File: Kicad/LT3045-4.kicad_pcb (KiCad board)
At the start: 4 copper layers, 100 x 50 mm, 26 parts, among them J1 Conn_Coaxial_Power, J2 Conn_Coaxial_Power, U1 LT3042, U2 LT3042, U3 LT3042, U4 LT3042

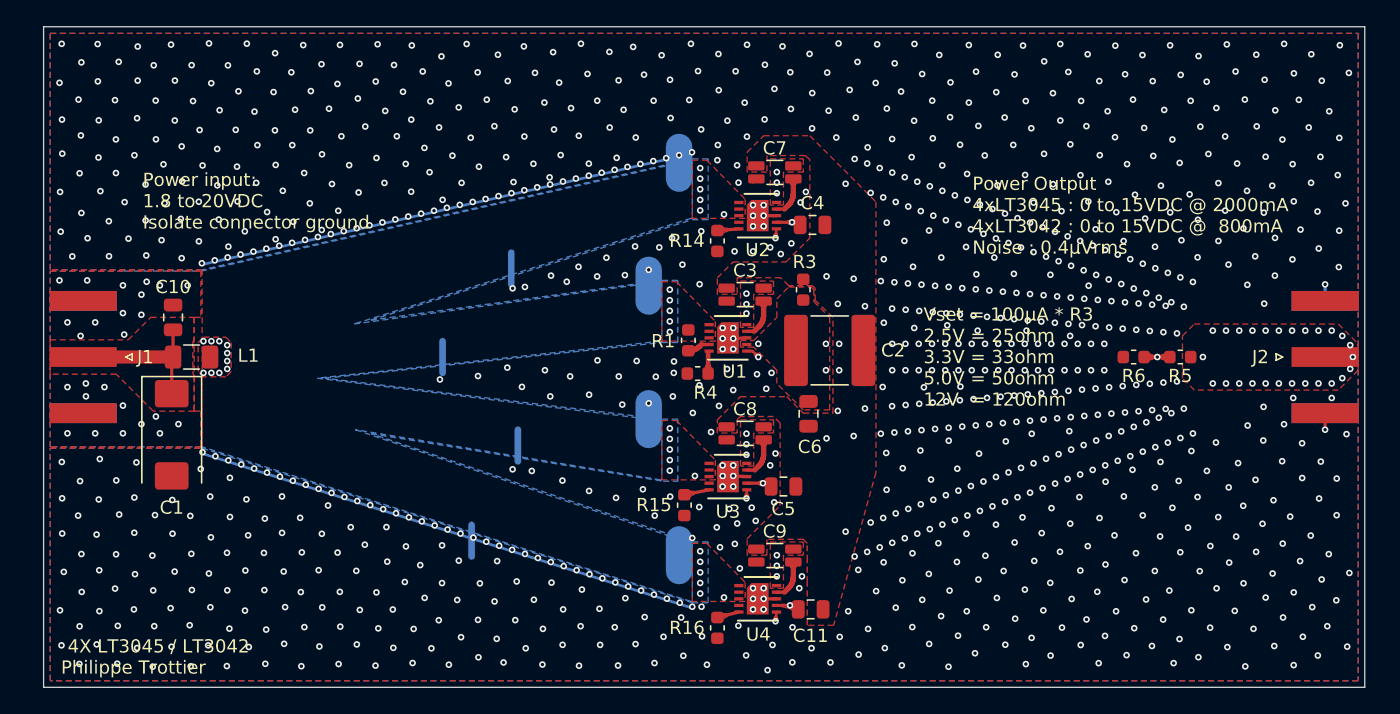
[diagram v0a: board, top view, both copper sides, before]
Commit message: Lost revision :(
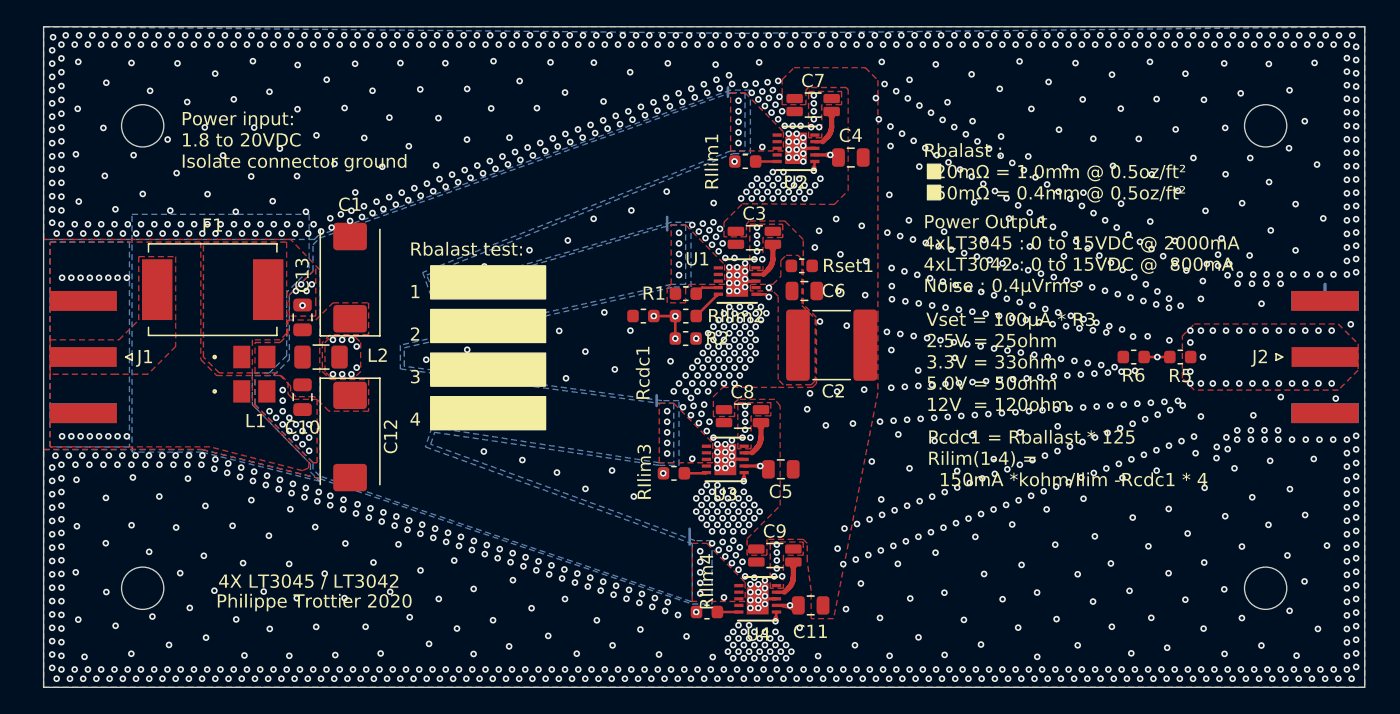
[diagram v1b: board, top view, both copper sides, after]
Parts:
- added C12: 22µF 35V, Capacitor_Tantalum_SMD:CP_EIA-7343-30_AVX-N, F.Cu at (23.2, 31.0)
- added C13: 4.7µF 35V, Capacitor_SMD:C_0805_2012Metric, F.Cu at (19.6, 22.0)
- added F1: 4A, Fuse:Fuse_Bourns_MF-SM_9.5x6.71mm, F.Cu at (12.8, 19.9)
- added L1: DLW5BTH101TQ2L, Transformer_SMD:CMC_DLW5BTH, F.Cu at (15.9, 26.3)
- added MH1: MountingHole_Pad, MountingHole:MountingHole_3.2mm_M3, F.Cu at (92.5, 7.50)
- added MH2: MountingHole_Pad, MountingHole:MountingHole_3.2mm_M3, F.Cu at (92.5, 42.5)
- added MH3: MountingHole_Pad, MountingHole:MountingHole_3.2mm_M3, F.Cu at (7.50, 7.50)
- added MH4: MountingHole_Pad, MountingHole:MountingHole_3.2mm_M3, F.Cu at (7.50, 42.5)
- added R2: 16.5k, Resistor_SMD:R_0603_1608Metric, F.Cu at (48.6, 23.6)
- added Rcdc1: Rcdc, Resistor_SMD:R_0603_1608Metric, F.Cu at (45.4, 21.9)
- RIlim1: renamed from R14; value 0 -> 287
- RIlim2: renamed from R4; value 0 -> 287
- RIlim3: renamed from R15; value 0 -> 287
- RIlim4: renamed from R16; value 0 -> 287
- moved C1 18.0 mm to (23.2, 19.0), turned to 90 degrees
- moved C10 11.5 mm to (19.6, 28.0), turned to 270 degrees
- moved L2 9.80 mm to (21.0, 25.0)
- moved C6 9.31 mm to (57.6, 20.0), turned to 0 degrees
- moved RIlim1 6.37 mm to (53.1, 10.2), turned to 180 degrees
- moved U2 5.87 mm to (57.0, 9.20)
- moved C7 5.87 mm to (58.2, 5.92)
- moved C4 5.87 mm to (61.1, 9.90)
- moved RIlim2 4.44 mm to (48.6, 21.9)
- moved U1 4.36 mm to (52.5, 19.2)
- moved C3 4.36 mm to (53.8, 16.0)
- moved R1 3.54 mm to (48.6, 20.2), turned to 180 degrees
- moved RIlim3 2.54 mm to (47.7, 33.8), turned to 180 degrees
- moved Rset1 1.80 mm to (57.4, 18.1), turned to 0 degrees
- moved RIlim4 1.44 mm to (50.2, 44.3), turned to 180 degrees
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- renumbered L1 to L2, R3 to Rset1
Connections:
- J1 pad 1: Net-(C1-Pad1) -> Net-(F1-Pad2)
- J1 pad 2: GND -> Net-(J1-Pad2)
- RIlim1 pad 2: GND -> /ILim
- RIlim2 pad 2: GND -> /ILim
- RIlim3 pad 2: GND -> /ILim
- RIlim4 pad 2: GND -> /ILim
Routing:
- net GND: track 105.6 -> 9.51 mm, vias 1093 -> 1604
- net /ILim: track 0.00 -> 41.6 mm, vias 0 -> 6
- net Net-(C1-Pad1): track 11.7 -> 0.00 mm
- net /VOUT: track 141.8 -> 131.5 mm, vias 38 -> 57
- net Net-(C11-Pad1): track 4.97 -> 12.7 mm, vias 4 -> 5
- net Net-(J1-Pad2): track 0.00 -> 2.39 mm, vias 0 -> 16
- net Net-(RIlim2-Pad1): track 1.73 -> 2.46 mm
- net /VIN: track 16.2 -> 15.8 mm, vias 36 -> 34
- added copper zone on In1.Cu, net /ILim
- added copper zone on F.Cu, net Net-(F1-Pad1)
- added copper zone on F.Cu, net Net-(F1-Pad2)
- added copper zone on B.Cu, net Net-(J1-Pad2)
- added copper zone on F.Cu, net Net-(J1-Pad2)
- added copper zone on In1.Cu, net Net-(J1-Pad2)
- added copper zone on In2.Cu, net Net-(J1-Pad2)
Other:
- board text added: "Pcdc1 = Rballast * 125 Rilim(1-4) = 150mA *kohm/Ilim -Rcdc1 * 4"
- board text added: "Philippe Trottier 2020"
- board text added: "Rbalast : 20mΩ = 1.0mm @ 0.5oz/ft² 50mΩ = 0.4mm @ 0.5oz/ft²"
- board text added: "Rbalast test: 1 mΩ 2 mΩ 3 mΩ 4 mΩ"
- board text removed: "Philippe Trottier"
